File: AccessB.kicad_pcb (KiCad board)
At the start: 2 copper layers, 50 x 50 mm, 30 parts, among them P1 ICSP, P2 USB_OTG, P3 GPIO, P5 USB_OTG, Q1 BSS138, Q2 BSS138, Q3 BSS138, Q4 BSS138, Q5 BSS138, U1 PIC18(L)F2550-I/SO, Y1 4MHz

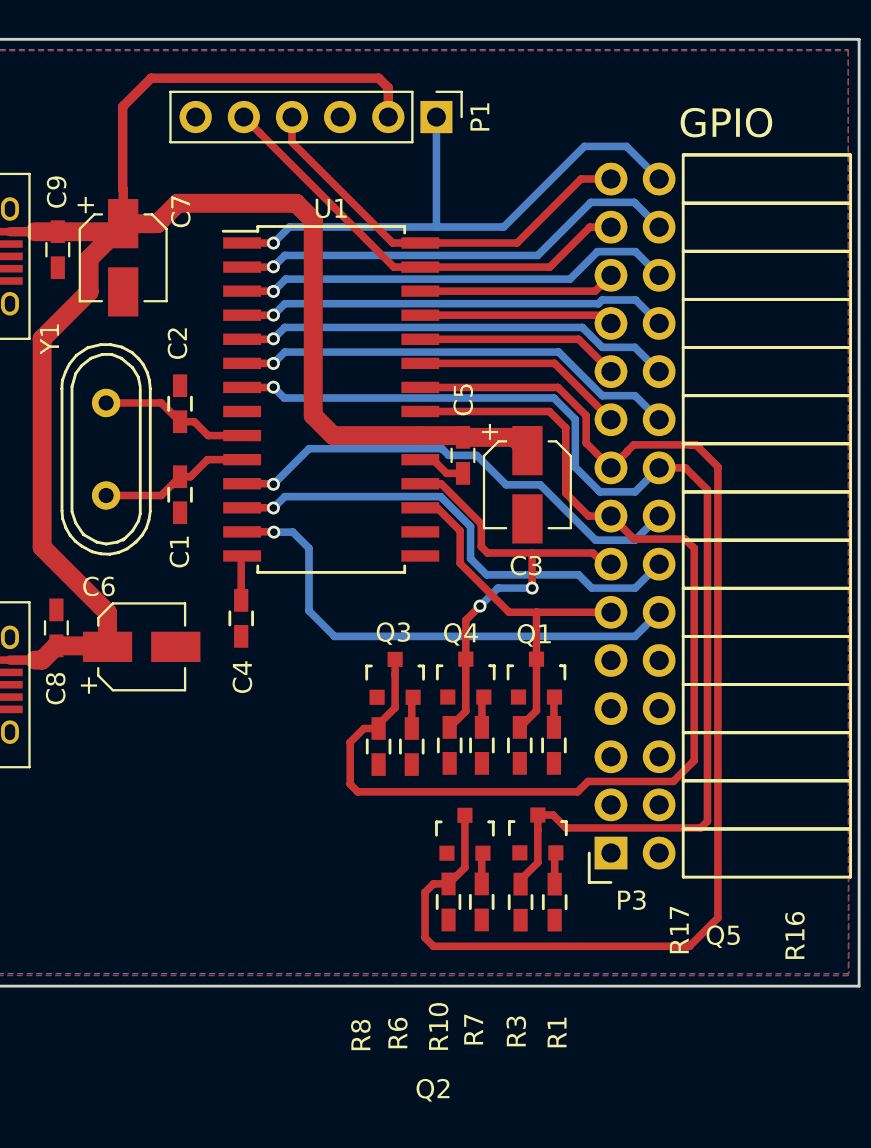
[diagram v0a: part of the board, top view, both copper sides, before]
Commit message: Update
Some reworking....
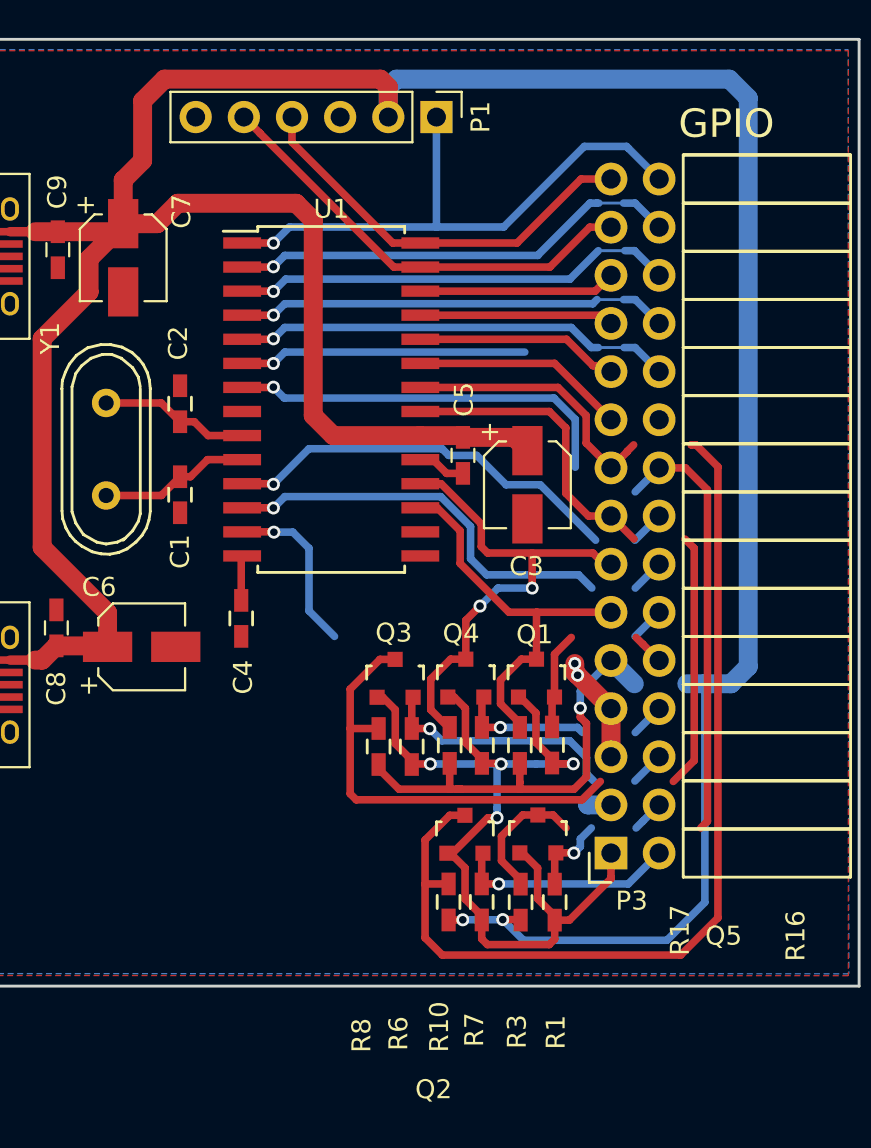
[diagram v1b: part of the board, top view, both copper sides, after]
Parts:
- moved R1 0.10 mm to (170.4, 106.7)
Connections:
- P2 pad 4: Net-(P2-Pad4) -> (no net)
- P3 pad 10: /GPIO11/RA5_VLS -> /GPIO4/RC6_VLS
- P3 pad 2: /GPIO5/RC7_VLS -> /GPIO13/RB1_VLS
- P3 pad 4: /GPIO4/RC6_VLS -> /GPIO11/RA5_VLS
- P3 pad 6: /GPIO13/RB1_VLS -> /GPIO12/RB0_VLS
- P3 pad 8: /GPIO12/RB0_VLS -> /GPIO5/RC7_VLS
- P5 pad 2: Net-(P5-Pad2) -> (no net)
- P5 pad 3: Net-(P5-Pad3) -> (no net)
- P5 pad 4: Net-(P5-Pad4) -> (no net)
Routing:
- net +5V: track 92.9 -> 198.5 mm, vias 0 -> 3
- net /VLS: track 0.00 -> 50.5 mm, vias 0 -> 4
- net /GPIO3/RC2: track 26.7 -> 10.9 mm
- net /GPIO12/RB0_VLS: track 1.68 -> 14.7 mm, vias 0 -> 1
- net /GPIO13/RB1_VLS: track 1.65 -> 11.7 mm, vias 0 -> 1
- net /GPIO11/RA5: track 60.2 -> 50.7 mm
- net /GPIO10/RA4: track 23.7 -> 15.2 mm
- net GND: track 2.55 -> 9.98 mm, vias 0 -> 2
- net /GPIO5/RC7_VLS: track 1.64 -> 8.84 mm, vias 0 -> 1
- net /GPIO4/RC6_VLS: track 1.61 -> 6.91 mm
- net /GPIO11/RA5_VLS: track 1.67 -> 6.05 mm, vias 0 -> 1
- net /GPIO12/RB0: track 57.7 -> 53.5 mm
- net /GPIO2/RC1: track 25.8 -> 23.5 mm
- net /GPIO1/RC0: track 25.3 -> 23.2 mm
- net /GPIO13/RB1: track 67.2 -> 65.8 mm
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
